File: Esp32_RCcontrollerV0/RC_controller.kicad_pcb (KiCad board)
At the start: 4 copper layers, 84 x 53 mm, 15 parts, among them J6 5V_Signal, U1 XL1509-5.0, U2 NODEMCU-32S, U4 BOB-12009, U5 BOB-12009

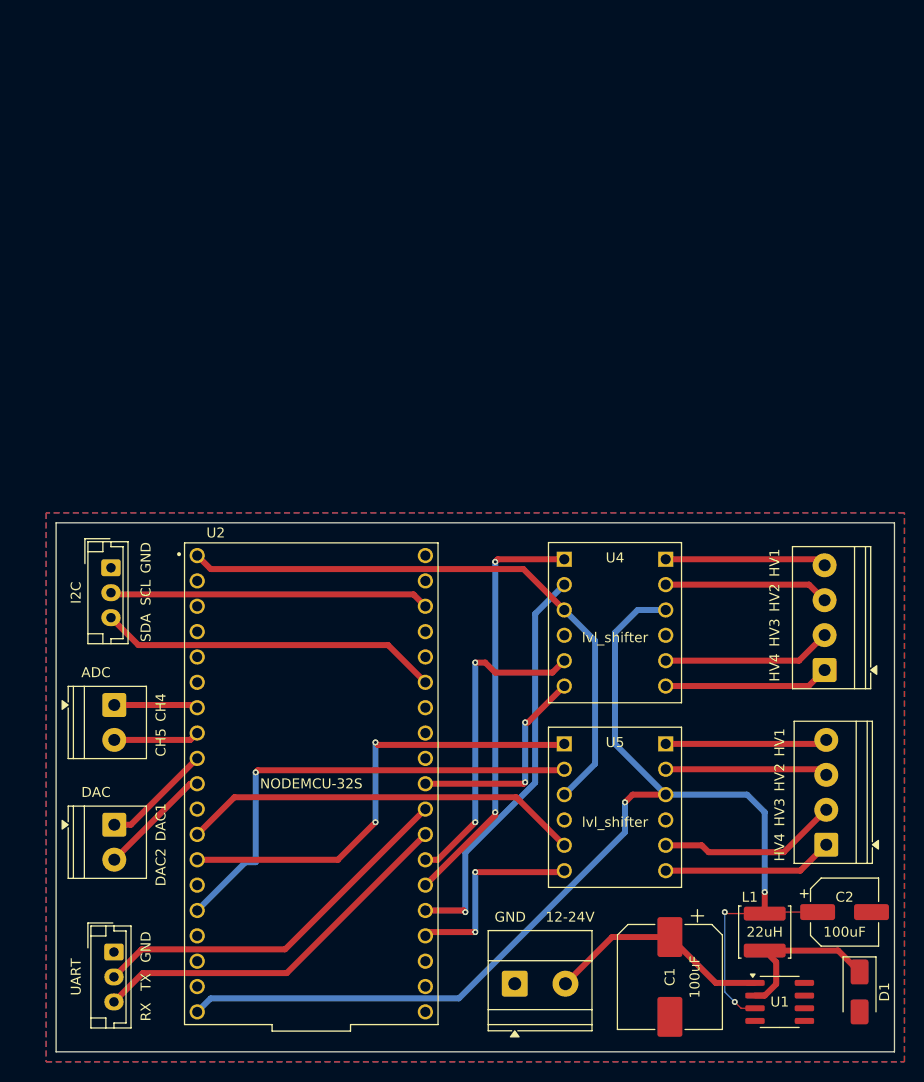
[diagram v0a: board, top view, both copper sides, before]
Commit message: Core updates
Rework the board , Added Doc
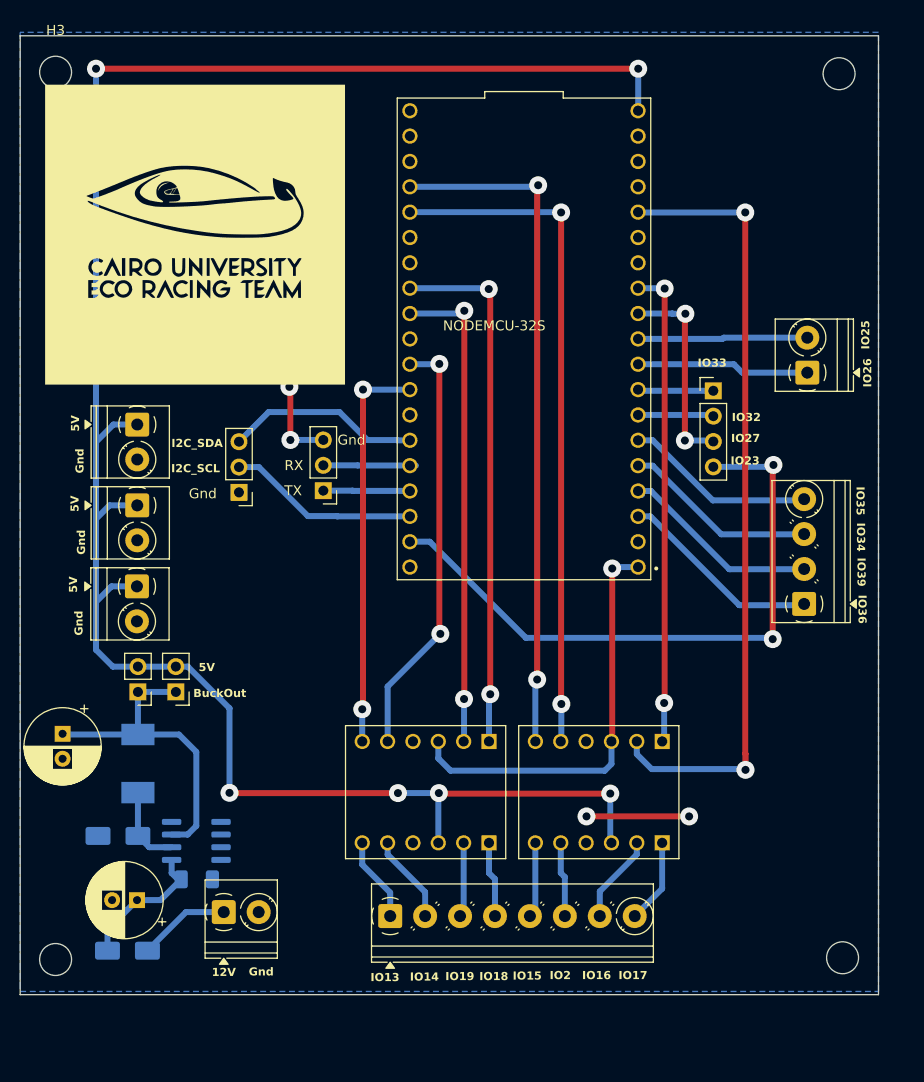
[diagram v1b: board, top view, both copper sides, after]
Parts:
- removed ADC, DAC: Conn_01x02_Socket, TerminalBlock_Phoenix:TerminalBlock_Phoenix_PT-1,5-2-3.5-H_1x02_P3.50mm_Horizontal
- removed GND: INPUT POWER (12 - 24V), TerminalBlock_Phoenix:TerminalBlock_Phoenix_MKDS-1,5-2-5.08_1x02_P5.08mm_Horizontal
- removed HV1: 5V_Signal, TerminalBlock_Phoenix:TerminalBlock_Phoenix_PT-1,5-4-3.5-H_1x04_P3.50mm_Horizontal
- removed U5: BOB-12009, BOB-12009:CONV_BOB-12009
- added C3: 10u, Capacitor_SMD:C_1206_3216Metric_Pad1.33x1.80mm_HandSolder, B.Cu at (106.1, 124.7)
- added D3: SS310, Diode_SMD:D_SMA, B.Cu at (99.2, 131.9)
- added G***: LOGO, LOGO, F.Cu at (105.9, 60.1)
- added H1: MountingHole, MountingHole:MountingHole_3.2mm_M3, F.Cu at (170.4, 44.0)
- added H2: MountingHole, MountingHole:MountingHole_3.2mm_M3, F.Cu at (170.8, 132.6)
- added H3: MountingHole, MountingHole:MountingHole_3.2mm_M3, F.Cu at (92.0, 43.9)
- added H4: MountingHole, MountingHole:MountingHole_3.2mm_M3, F.Cu at (92.0, 132.8)
- added J10: Screw_Terminal_01x02, TerminalBlock_Phoenix:TerminalBlock_Phoenix_PT-1,5-2-3.5-H_1x02_P3.50mm_Horizontal, F.Cu at (100.1, 87.2)
- added J3: Conn_01x04_Pin, Connector_PinHeader_2.54mm:PinHeader_1x04_P2.54mm_Vertical, F.Cu at (157.8, 75.8)
- added J4: Screw_Terminal_01x04, TerminalBlock_Phoenix:TerminalBlock_Phoenix_PT-1,5-4-3.5-H_1x04_P3.50mm_Horizontal, F.Cu at (166.9, 97.1)
- added J5: Digital I/O, TerminalBlock_Phoenix:TerminalBlock_Phoenix_PT-1,5-8-3.5-H_1x08_P3.50mm_Horizontal, F.Cu at (125.5, 128.4)
- added J7: DAC_OUT, TerminalBlock_Phoenix:TerminalBlock_Phoenix_PT-1,5-2-3.5-H_1x02_P3.50mm_Horizontal, F.Cu at (167.3, 74.0)
- added J8: Screw_Terminal_01x02, TerminalBlock_Phoenix:TerminalBlock_Phoenix_PT-1,5-2-3.5-H_1x02_P3.50mm_Horizontal, F.Cu at (100.1, 95.4)
- added J9: Screw_Terminal_01x02, TerminalBlock_Phoenix:TerminalBlock_Phoenix_PT-1,5-2-3.5-H_1x02_P3.50mm_Horizontal, F.Cu at (100.1, 79.2)
- added JP1: Jumper_2_Bridged, Connector_PinHeader_2.54mm:PinHeader_1x02_P2.54mm_Vertical, F.Cu at (100.2, 105.9)
- added JP2: Jumper_2_Bridged, Connector_PinHeader_2.54mm:PinHeader_1x02_P2.54mm_Vertical, F.Cu at (104.0, 105.9)
- added U3: BOB-12009, LibMain:CONV_BOB-12009, F.Cu at (129.0, 116.0)
- C1: value 100u -> 180u; footprint Capacitor_SMD:CP_Elec_10x10 -> Capacitor_THT:CP_Radial_D7.5mm_P2.50mm
- C2: footprint Capacitor_SMD:CP_Elec_6.3x5.8 -> Capacitor_THT:CP_Radial_D7.5mm_P2.50mm
- D1, U1: moved to B.Cu
- J1: renamed from UART; footprint Connector_JST:JST_EH_B3B-EH-A_1x03_P2.50mm_Vertical -> Connector_PinHeader_2.54mm:PinHeader_1x03_P2.54mm_Vertical
- J2: renamed from I2C; footprint Connector_JST:JST_EH_B3B-EH-A_1x03_P2.50mm_Vertical -> Connector_PinHeader_2.54mm:PinHeader_1x03_P2.54mm_Vertical
- J6: value 5V_Signal -> Screw_Terminal_01x02; footprint TerminalBlock_Phoenix:TerminalBlock_Phoenix_PT-1,5-4-3.5-H_1x04_P3.50mm_Horizontal -> TerminalBlock_Phoenix:TerminalBlock_Phoenix_PT-1,5-2-3.5-H_1x02_P3.50mm_Horizontal
- L1: value 22u -> 68uH; footprint Inductor_SMD:L_APV_ANR5020 -> EasyEDA:IND-SMD_L7.1-W6.6_H5.0; moved to B.Cu
- U2: footprint NODEMCU-32S:MODULE_NODEMCU-32S -> LibMain:MODULE_NODEMCU-32S
- U4: footprint BOB-12009:CONV_BOB-12009 -> LibMain:CONV_BOB-12009
- moved C2 80.4 mm to (92.7, 110.1), turned to -90 degrees
- moved D1 75.9 mm to (98.2, 120.4), turned to 180 degrees
- moved L1 65.0 mm to (100.2, 113.1)
- moved J6 60.7 mm to (108.8, 128.0), turned to 0 degrees
- moved U1 60.6 mm to (106.0, 120.9)
- moved C1 53.9 mm to (100.1, 126.8), turned to 180 degrees
- moved J1 50.8 mm to (118.8, 85.8), turned to 180 degrees
- moved U2 49.4 mm to (138.9, 70.6), turned to 180 degrees
- moved U4 17.1 mm to (146.4, 116.0), turned to -90 degrees
- moved J2 14.9 mm to (110.3, 86.0), turned to 180 degrees
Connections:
- net Net-(J2-Pin_2) renamed /I2C_SCL
- net Net-(J2-Pin_3) renamed /I2C_SDA
- C2 pad 1: 5V -> Net-(JP1-A)
- J1 pad 1: GND -> Net-(J1-Pin_1)
- J1 pad 3: Net-(J1-Pin_3) -> GND
- J6 pad 2: Net-(J6-Pin_2) -> GND
- L1 pad 2: 5V -> Net-(JP1-A)
- U1 pad 3: 5V -> Net-(JP1-A)
- U2 pad J1_11: unconnected-(U2-IO27-PadJ1_11) -> Net-(J3-Pin_3)
- U2 pad J1_12: LV_Signal7 -> IO14_LowLogic
- U2 pad J1_13: LV_Signal5 -> unconnected-(U2-IO12-PadJ1_13)
- U2 pad J1_15: LV_Signal6 -> IO13_LowLogic
- U2 pad J1_19: 5V -> +5V
- U2 pad J1_3: unconnected-(U2-IO36-PadJ1_3) -> /IO36
- U2 pad J1_4: unconnected-(U2-IO39-PadJ1_4) -> /IO39
- U2 pad J1_5: unconnected-(U2-IO34-PadJ1_5) -> /IO34
- U2 pad J1_6: unconnected-(U2-IO35-PadJ1_6) -> /IO35
- U2 pad J2_10: LV_Signal4 -> unconnected-(U2-IO5-PadJ2_10)
- U2 pad J2_11: Net-(J1-Pin_2) -> IO17_LowLogic
- U2 pad J2_12: Net-(J1-Pin_3) -> IO16_LowLogic
- U2 pad J2_13: LV_Signal3 -> unconnected-(U2-IO4-PadJ2_13)
- U2 pad J2_14: LV_Signal1 -> unconnected-(U2-IO0-PadJ2_14)
- U2 pad J2_15: LV_Signal2 -> IO2_LowLogic
- U2 pad J2_16: LV_Signal8 -> IO15_LowLogic
- U2 pad J2_2: unconnected-(U2-IO23-PadJ2_2) -> Net-(J3-Pin_4)
- U2 pad J2_4: unconnected-(U2-TX0-PadJ2_4) -> Net-(J1-Pin_1)
- U2 pad J2_5: unconnected-(U2-RX0-PadJ2_5) -> Net-(J1-Pin_2)
- U2 pad J2_8: unconnected-(U2-IO19-PadJ2_8) -> IO19_LowLogic
- U2 pad J2_9: unconnected-(U2-IO18-PadJ2_9) -> IO18_LowLogic
- U4 pad HV: 5V -> +5V
- U4 pad HV1: Net-(J5-Pin_4) -> IO17_HighLogic
- U4 pad HV2: Net-(J5-Pin_3) -> IO16_HighLogic
- U4 pad HV3: Net-(J5-Pin_2) -> IO2_HighLogic
- U4 pad HV4: Net-(J5-Pin_1) -> IO15_HighLogic
- U4 pad LV1: LV_Signal1 -> IO14_LowLogic
- U4 pad LV2: LV_Signal2 -> IO13_LowLogic
- U4 pad LV3: LV_Signal3 -> IO2_LowLogic
- U4 pad LV4: LV_Signal4 -> IO15_LowLogic
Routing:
- net +5V: track 0.00 -> 204.7 mm, vias 0 -> 6
- net 5V: track 124.0 -> 0.00 mm, vias 4 -> 0
- net IO13_LowLogic: track 0.00 -> 79.4 mm, vias 0 -> 2
- net IO15_LowLogic: track 0.00 -> 68.8 mm, vias 0 -> 2
- net IO2_LowLogic: track 0.00 -> 68.2 mm, vias 0 -> 2
- net Net-(J3-Pin_4): track 0.00 -> 64.0 mm, vias 0 -> 2
- net IO16_LowLogic: track 0.00 -> 53.4 mm, vias 0 -> 2
- net IO17_LowLogic: track 0.00 -> 48.7 mm, vias 0 -> 2
- net IO14_LowLogic: track 0.00 -> 48.2 mm, vias 0 -> 2
- net LV_Signal6: track 47.9 -> 0.00 mm, vias 1 -> 0
- net LV_Signal5: track 46.5 -> 0.00 mm, vias 2 -> 0
- net IO18_LowLogic: track 0.00 -> 43.0 mm, vias 0 -> 2
- net LV_Signal1: track 42.3 -> 0.00 mm, vias 2 -> 0
- net LV_Signal2: track 41.0 -> 0.00 mm, vias 1 -> 0
- net LV_Signal7: track 40.3 -> 0.00 mm
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- removed copper zone on F.Cu, net GND
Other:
- board size 84 x 53 mm -> 86 x 96.1 mm
- copper layers 4 -> 2
- board text added: "12V"
- board text added: "5V"
- board text added: "BuckOut"
- board text added: "Gnd"
- board text added: "I2C_SCL"
- board text added: "I2C_SDA"
- board text added: "IO13"
- board text added: "IO14"
- board text added: "IO15"
- board text added: "IO16"
- board text added: "IO17"
- board text added: "IO18"
- board text added: "IO19"
- board text added: "IO2"
- board text added: "IO23"
- board text added: "IO25"
- board text added: "IO26"
- board text added: "IO27"
- board text added: "IO32"
- board text added: "IO33"
- board text added: "IO34"
- board text added: "IO35"
- board text added: "IO36"
- board text added: "IO39"
- board text removed: "100uF"
- board text removed: "12-24V"
- board text removed: "22uH"
- board text removed: "CH4"
- board text removed: "CH5"
- board text removed: "DAC1"
- board text removed: "DAC2"
- board text removed: "GND"
- board text removed: "HV1"
- board text removed: "HV2"
- board text removed: "HV3"
- board text removed: "HV4"
- board text removed: "L1"
- board text removed: "SCL"
- board text removed: "SDA"
- board text removed: "lvl_shifter"
